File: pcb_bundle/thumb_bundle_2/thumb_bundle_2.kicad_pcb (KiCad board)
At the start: 2 copper layers, 98.7 x 100.2 mm, 53 parts

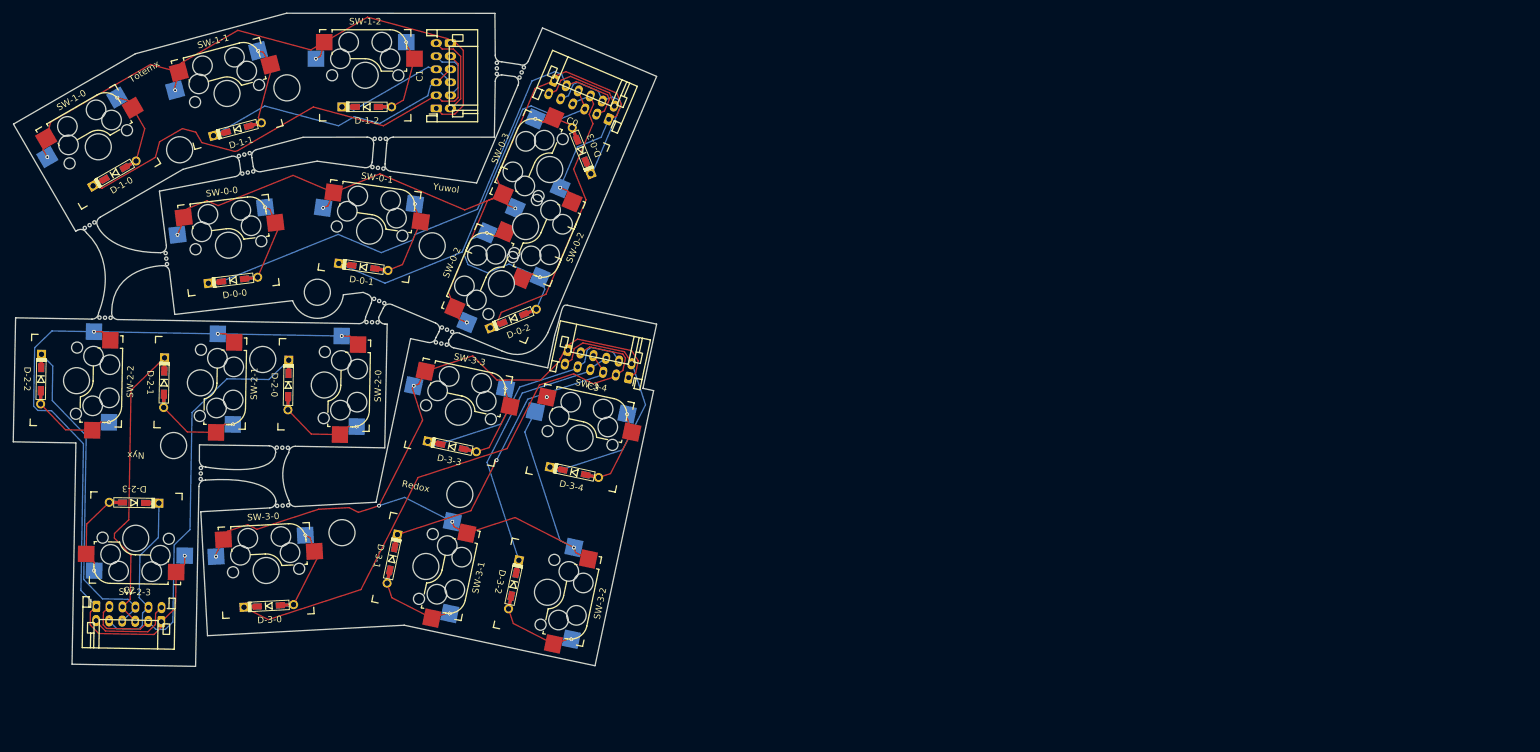
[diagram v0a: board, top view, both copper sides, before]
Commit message: [unstable] interim state
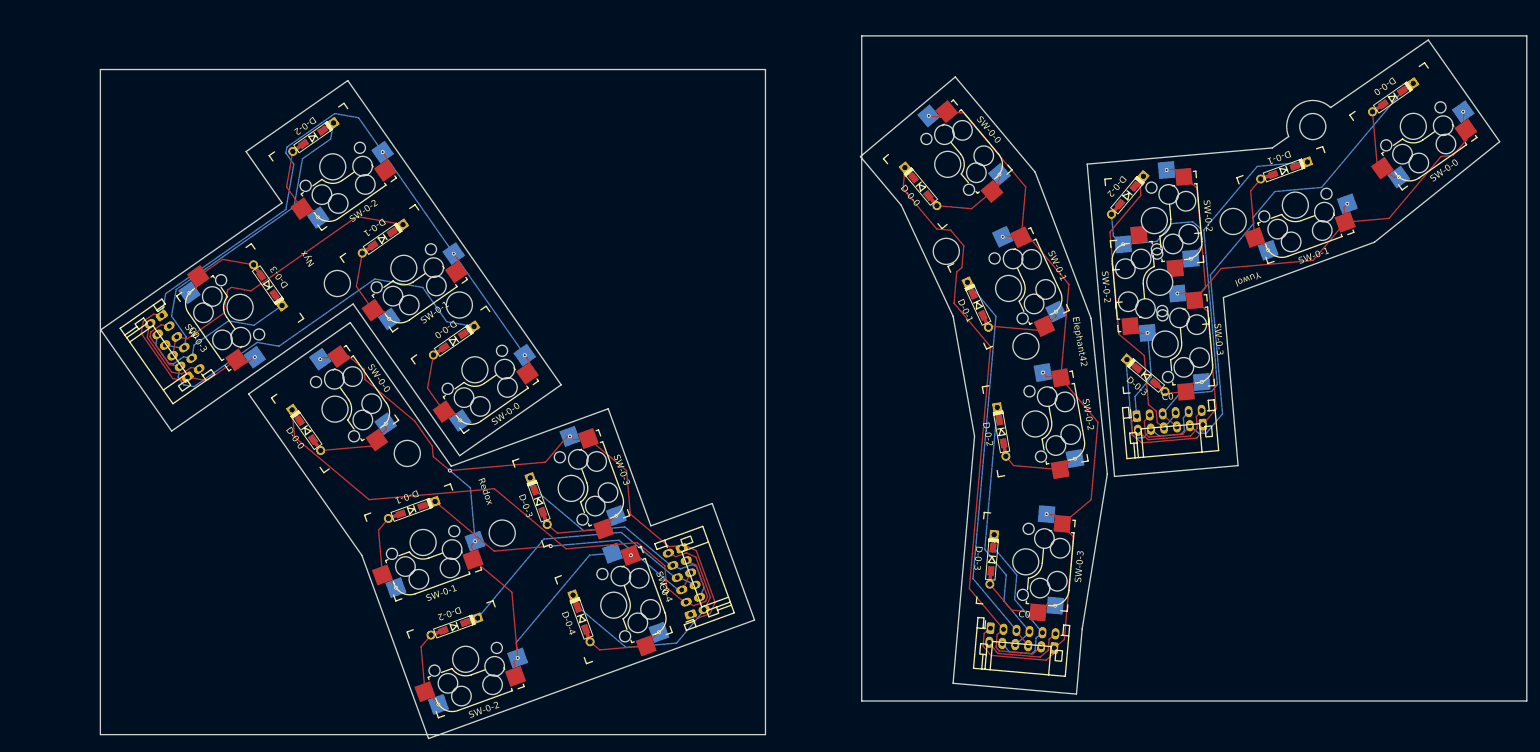
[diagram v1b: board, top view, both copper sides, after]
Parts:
- removed the C0 at (106.7, 39.7)
- removed C1, C2, C3: Conn_01x06_Socket, crustrusk:reversible JST_PH_S6B-PH-K_1x06_P2.00mm_Horizontal
- removed the D-0-0 at (49.0, 64.4)
- removed the D-0-1 at (69.0, 62.3)
- removed the D-0-2 at (92.0, 70.2)
- removed the D-0-3 at (102.5, 44.5)
- removed D-1-0, D-1-1, D-1-2, D-2-0, D-2-1, D-2-2, D-2-3, D-3-0, D-3-1, D-3-2, D-3-3, D-3-4: D, crustrusk:Diode_TH_SMD_REVERSIBLE
- removed REF** (x16): MouseBite-Part_2.0x2.0mm_outset_D0.5mm_P0.85mm_3h, Panelization:MouseBite-Part_2.0x2.0mm_outset_D0.5mm_P0.85mm_3h
- removed the SW-0-0 at (48.3, 59.0)
- removed the SW-0-1 at (70.0, 56.8)
- removed the SW-0-2 at (90.2, 64.9)
- removed the SW-0-2 at (93.9, 56.1)
- removed the SW-0-3 at (97.6, 47.4)
- removed SW-1-0, SW-1-1, SW-1-2, SW-2-0, SW-2-1, SW-2-2, SW-2-3, SW-3-0, SW-3-1, SW-3-2, SW-3-3, SW-3-4: SW_Push, crustrusk:Kailh_hotswap_only_socket_MX_optional_reversible-MIRROR
- added C0: Conn_01x06_Socket, crustrusk:reversible JST_PH_S6B-PH-K_1x06_P2.00mm_Horizontal, F.Cu at (38.1, 69.8)
- added C0: Conn_01x06_Socket, crustrusk:reversible JST_PH_S6B-PH-K_1x06_P2.00mm_Horizontal, F.Cu at (119.2, 115.6)
- added C0: Conn_01x06_Socket, crustrusk:reversible JST_PH_S6B-PH-K_1x06_P2.00mm_Horizontal, F.Cu at (165.2, 117.7)
- added C0: Conn_01x06_Socket, crustrusk:reversible JST_PH_S6B-PH-K_1x06_P2.00mm_Horizontal, F.Cu at (187.6, 85.2)
- added D-0-0: D, crustrusk:Diode_TH_SMD_REVERSIBLE, F.Cu at (82.9, 73.6)
- added D-0-0: D, crustrusk:Diode_TH_SMD_REVERSIBLE, F.Cu at (60.3, 87.4)
- added D-0-0: D, crustrusk:Diode_TH_SMD_REVERSIBLE, F.Cu at (154.5, 50.0)
- added D-0-0: D, crustrusk:Diode_TH_SMD_REVERSIBLE, F.Cu at (226.9, 36.4)
- added D-0-1: D, crustrusk:Diode_TH_SMD_REVERSIBLE, F.Cu at (163.3, 68.1)
- added D-0-1: D, crustrusk:Diode_TH_SMD_REVERSIBLE, F.Cu at (72.0, 58.0)
- added D-0-1: D, crustrusk:Diode_TH_SMD_REVERSIBLE, F.Cu at (210.2, 47.5)
- added D-0-1: D, crustrusk:Diode_TH_SMD_REVERSIBLE, F.Cu at (76.4, 99.6)
- added D-0-2: D, crustrusk:Diode_TH_SMD_REVERSIBLE, F.Cu at (166.9, 87.6)
- added D-0-2: D, crustrusk:Diode_TH_SMD_REVERSIBLE, F.Cu at (61.3, 42.4)
- added D-0-2: D, crustrusk:Diode_TH_SMD_REVERSIBLE, F.Cu at (186.2, 51.3)
- added D-0-2: D, crustrusk:Diode_TH_SMD_REVERSIBLE, F.Cu at (83.0, 117.5)
- added D-0-3: D, crustrusk:Diode_TH_SMD_REVERSIBLE, F.Cu at (189.0, 79.0)
- added D-0-3: D, crustrusk:Diode_TH_SMD_REVERSIBLE, F.Cu at (165.4, 107.2)
- added D-0-3: D, crustrusk:Diode_TH_SMD_REVERSIBLE, F.Cu at (54.4, 65.1)
- added D-0-3: D, crustrusk:Diode_TH_SMD_REVERSIBLE, F.Cu at (95.9, 98.3)
- added D-0-4: D, crustrusk:Diode_TH_SMD_REVERSIBLE, F.Cu at (102.5, 116.2)
- added SW-0-0: SW_Push, crustrusk:Kailh_hotswap_only_socket_MX_optional_reversible-MIRROR, F.Cu at (64.7, 84.1)
- added SW-0-0: SW_Push, crustrusk:Kailh_hotswap_only_socket_MX_optional_reversible-MIRROR, F.Cu at (158.6, 46.6)
- added SW-0-0: SW_Push, crustrusk:Kailh_hotswap_only_socket_MX_optional_reversible-MIRROR, F.Cu at (86.1, 78.1)
- added SW-0-0: SW_Push, crustrusk:Kailh_hotswap_only_socket_MX_optional_reversible-MIRROR, F.Cu at (230.1, 40.8)
- added SW-0-1: SW_Push, crustrusk:Kailh_hotswap_only_socket_MX_optional_reversible-MIRROR, F.Cu at (75.2, 62.5)
- added SW-0-1: SW_Push, crustrusk:Kailh_hotswap_only_socket_MX_optional_reversible-MIRROR, F.Cu at (78.2, 104.6)
- added SW-0-1: SW_Push, crustrusk:Kailh_hotswap_only_socket_MX_optional_reversible-MIRROR, F.Cu at (212.0, 52.8)
- added SW-0-1: SW_Push, crustrusk:Kailh_hotswap_only_socket_MX_optional_reversible-MIRROR, F.Cu at (168.0, 65.6)
- added SW-0-2: SW_Push, crustrusk:Kailh_hotswap_only_socket_MX_optional_reversible-MIRROR, F.Cu at (84.7, 122.5)
- added SW-0-2: SW_Push, crustrusk:Kailh_hotswap_only_socket_MX_optional_reversible-MIRROR, F.Cu at (172.1, 86.4)
- added SW-0-2: SW_Push, crustrusk:Kailh_hotswap_only_socket_MX_optional_reversible-MIRROR, F.Cu at (64.3, 47.0)
- added SW-0-2: SW_Push, crustrusk:Kailh_hotswap_only_socket_MX_optional_reversible-MIRROR, F.Cu at (190.3, 55.2)
- added SW-0-2: SW_Push, crustrusk:Kailh_hotswap_only_socket_MX_optional_reversible-MIRROR, F.Cu at (191.2, 64.7)
- added SW-0-3: SW_Push, crustrusk:Kailh_hotswap_only_socket_MX_optional_reversible-MIRROR, F.Cu at (50.1, 68.5)
- added SW-0-3: SW_Push, crustrusk:Kailh_hotswap_only_socket_MX_optional_reversible-MIRROR, F.Cu at (100.9, 96.3)
- added SW-0-3: SW_Push, crustrusk:Kailh_hotswap_only_socket_MX_optional_reversible-MIRROR, F.Cu at (192.0, 74.2)
- added SW-0-3: SW_Push, crustrusk:Kailh_hotswap_only_socket_MX_optional_reversible-MIRROR, F.Cu at (170.6, 107.6)
- added SW-0-4: SW_Push, crustrusk:Kailh_hotswap_only_socket_MX_optional_reversible-MIRROR, F.Cu at (107.4, 114.2)
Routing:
- net COL0: track 140.0 -> 550.0 mm, vias 5 -> 19
- net ROW0-0: track 84.1 -> 328.8 mm
- net COL3: track 156.7 -> 0.00 mm, vias 6 -> 0
- net ROW1-0: track 57.4 -> 209.7 mm, vias 0 -> 1
- net ROW2-0: track 46.3 -> 177.8 mm
- net COL2: track 129.9 -> 0.00 mm, vias 4 -> 0
- net COL1: track 96.4 -> 0.00 mm, vias 3 -> 0
- net ROW3-0: track 24.3 -> 114.7 mm
- net ROW0-3: track 87.2 -> 0.00 mm
- net ROW0-1: track 71.7 -> 0.00 mm
- net ROW0-2: track 66.8 -> 0.00 mm
- net ROW4-0: track 13.2 -> 78.9 mm
- net ROW2-2: track 49.9 -> 0.00 mm
- net ROW1-3: track 46.3 -> 0.00 mm, vias 1 -> 0
- net ROW1-2: track 45.7 -> 0.00 mm
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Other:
- board size 98.7 x 100.2 mm -> 218.8 x 107.8 mm
- board text added: "Elephant42"
- board text removed: "Totemx"
